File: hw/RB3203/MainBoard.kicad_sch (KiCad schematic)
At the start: 8 parts

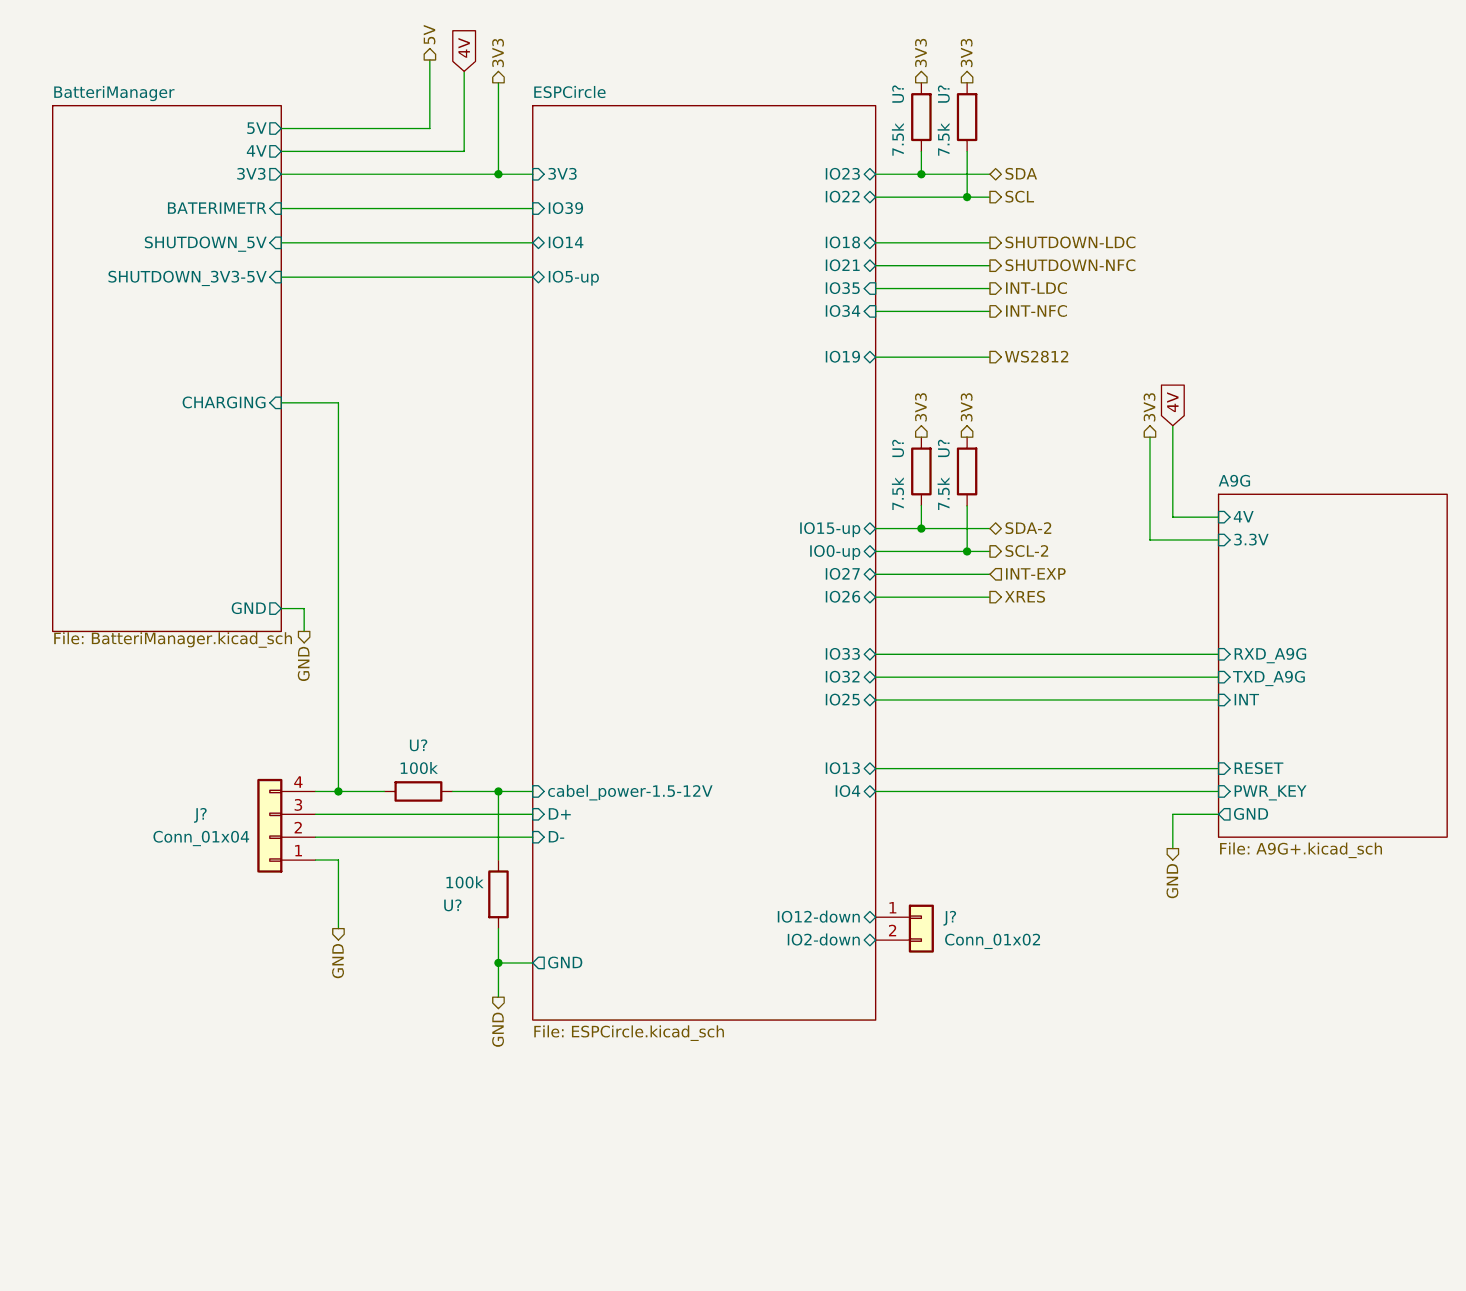
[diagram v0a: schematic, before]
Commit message: Wip
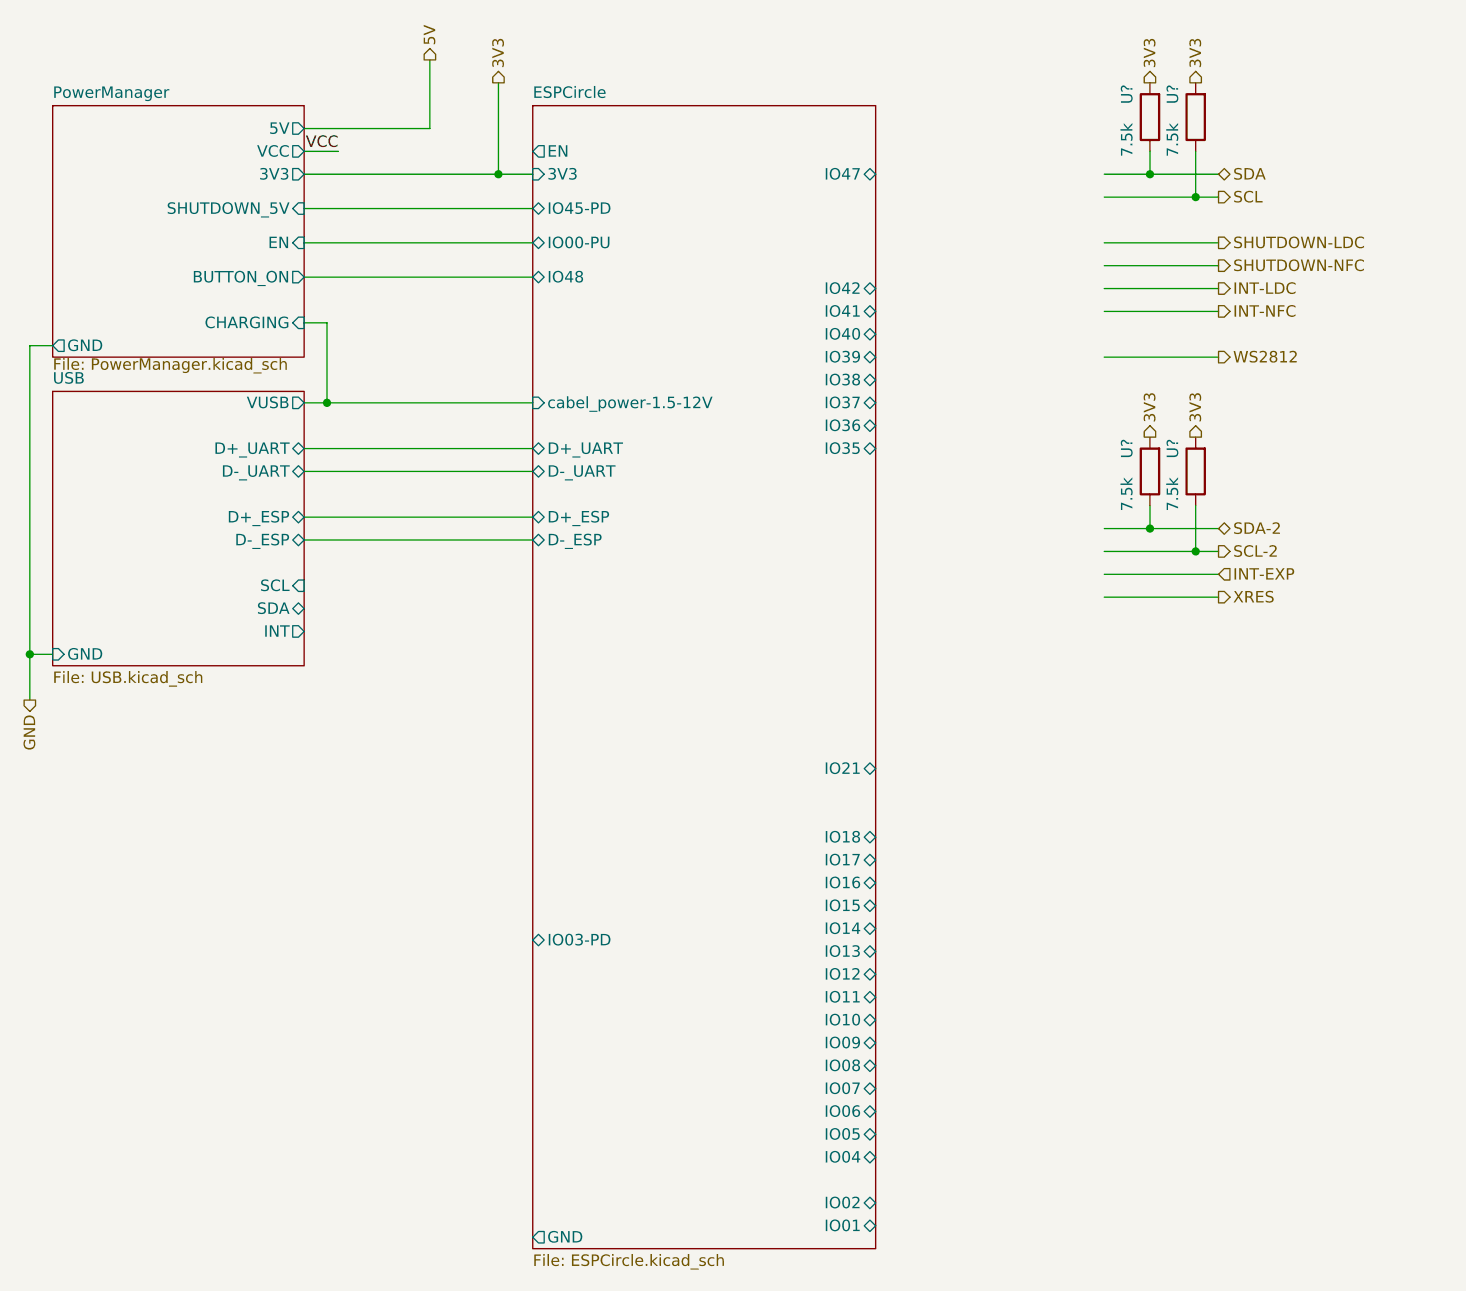
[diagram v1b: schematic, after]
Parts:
- removed J?: Conn_01x04, symbol Connector_Generic:Conn_01x04
- removed J?: Conn_01x02, symbol Connector_Generic:Conn_01x02
- removed U? (x2): 100k, Resistor_SMD:R_0402_1005Metric, symbol B.B-rescue:R-Device-B.B-rescue-B.B-rescue
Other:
- sheet BatteriManager renamed PowerManager
- removed sheet A9G
- added sheet USB (USB.kicad_sch)
- sheet ESPCircle ports: added D+_ESP, D+_UART, D-_ESP, D-_UART, EN, IO00-PU, IO01, IO02, IO03-PD, IO04, IO05, IO06, IO07, IO08, IO09, IO10, IO11, IO12, IO15, IO16, IO17, IO36, IO37, IO38, IO40, IO41, IO42, IO45-PD, IO47, IO48; removed D+, D-, IO0-up, IO12-down, IO15-up, IO19, IO2-down, IO22, IO23, IO25, IO26, IO27, IO32, IO33, IO34, IO4, IO5-up
- sheet PowerManager: file BatteriManager.kicad_sch -> PowerManager.kicad_sch
- sheet PowerManager ports: added BUTTON_ON, EN, VCC; removed 4V, BATERIMETR, SHUTDOWN_3V3-5V
- moved on the sheet: U?
